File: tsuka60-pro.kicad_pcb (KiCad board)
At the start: 2 copper layers, 285 x 94.6 mm, 171 parts, among them J1 USB_C_Receptacle_USB2.0, J2 Conn_01x04_MountingPin, SW1 SW_Reset, U1 ATmega32U4-M, U2 SRV05-4, Y1 16MHz

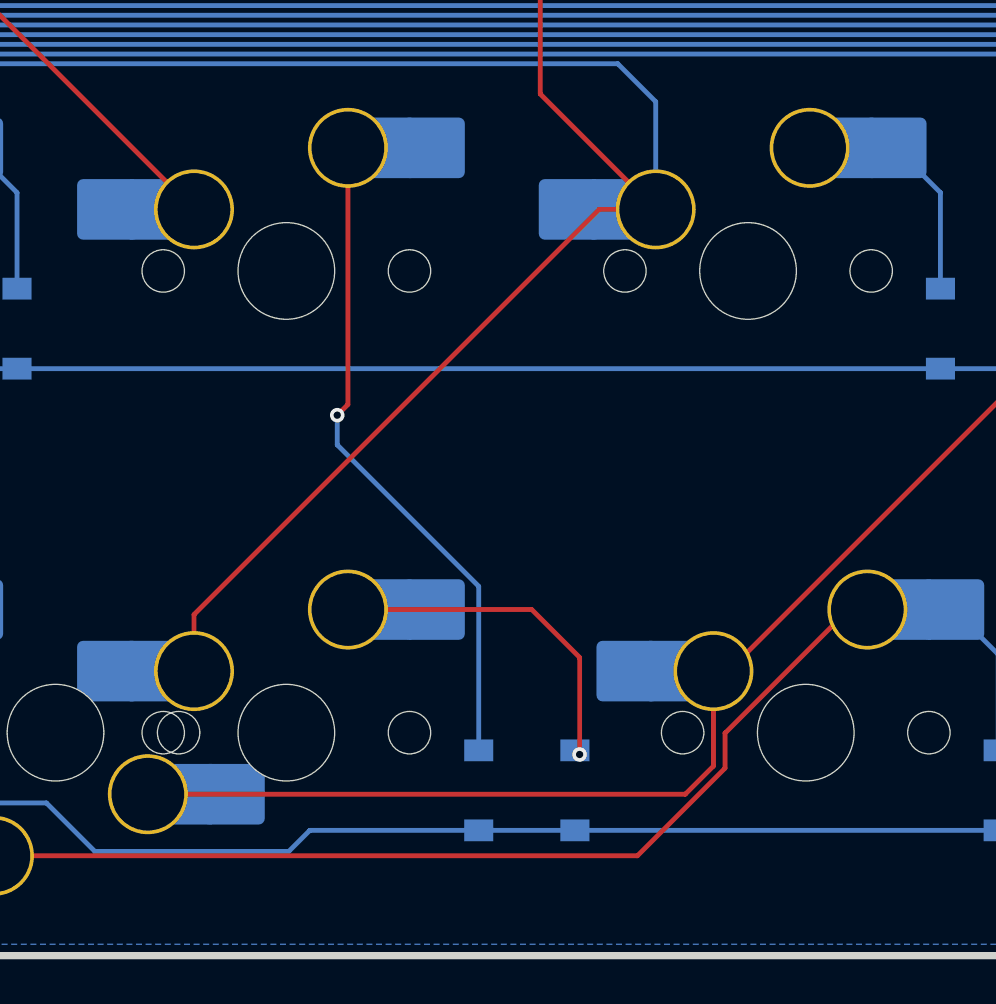
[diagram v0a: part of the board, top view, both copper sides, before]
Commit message: Update some traces
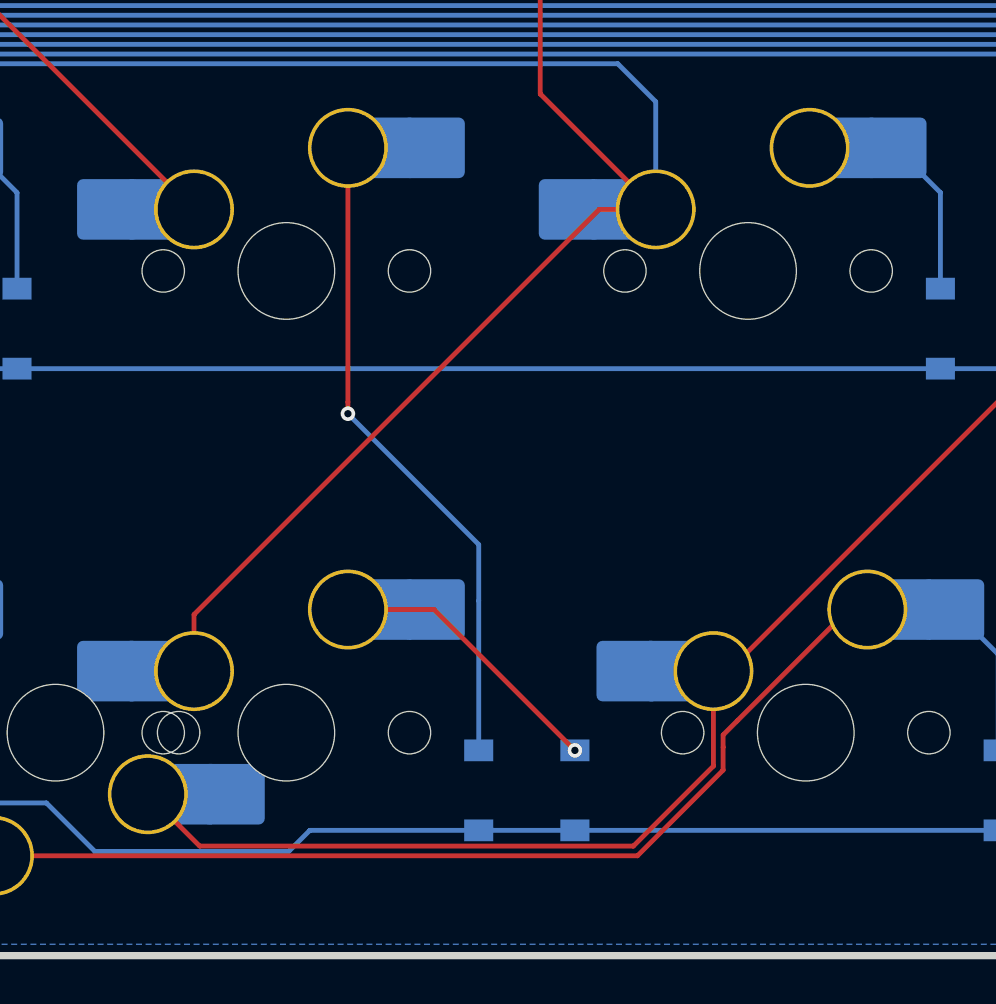
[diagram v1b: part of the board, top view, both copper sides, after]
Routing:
- net Net-(D69-Pad2): track 14.6 -> 11.8 mm
- net COL9: track 294.7 -> 296.4 mm
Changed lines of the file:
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@@
   (segment (start 187.325 161.922183) (end 187.325 165.83125) (width 0.2) (layer "B.Cu") (net 65))
   (segment (start 199.39 160.02) (end 189.227183 160.02) (width 0.2) (layer "B.Cu") (net 65))
-  (segment (start 218.44 151.56) (end 218 152) (width 0.2) (layer "F.Cu") (net 66))
-  (segment (start 218.44 140.97) (end 218.44 151.56) (width 0.2) (layer "F.Cu") (net 66))
-  (via (at 218 152) (size 0.6) (drill 0.3) (layers "F.Cu" "B.Cu") (net 66))
-  (segment (start 223.8375 165.83125) (end 223.8375 159.064683) (width 0.2) (layer "B.Cu") (net 66))
-  (segment (start 223.8375 159.064683) (end 218 153.227183) (width 0.2) (layer "B.Cu") (net 66))
-  (segment (start 218 153.227183) (end 218 152) (width 0.2) (layer "B.Cu") (net 66))
-  (segment (start 228 162) (end 226.02 160.02) (width 0.2) (layer "F.Cu") (net 67))
-  (segment (start 228 166) (end 228 162) (width 0.2) (layer "F.Cu") (net 67))
-  (segment (start 226.02 160.02) (end 218.44 160.02) (width 0.2) (layer "F.Cu") (net 67))
-  (via (at 228 166) (size 0.6) (drill 0.3) (layers "F.Cu" "B.Cu") (net 67))
-  (segment (start 227.83125 165.83125) (end 228 166) (width 0.2) (layer "B.Cu") (net 67))
-  (segment (start 227.80625 165.83125) (end 227.83125 165.83125) (width 0.2) (layer "B.Cu") (net 67))
+  (segment (start 218.44 140.97) (end 218.44 151.46) (width 0.2) (layer "F.Cu") (net 66))
+  (segment (start 218.44 151.46) (end 218.44 151.94) (width 0.2) (layer "F.Cu") (net 66))
+  (via (at 218.44 151.94) (size 0.6) (drill 0.3) (layers "F.Cu" "B.Cu") (net 66))
+  (segment (start 223.8375 165.83125) (end 223.8375 159.6625) (width 0.2) (layer "B.Cu") (net 66))
+  (segment (start 223.8375 157.3375) (end 218.44 151.94) (width 0.2) (layer "B.Cu") (net 66))
+  (segment (start 223.8375 159.6625) (end 223.8375 157.3375) (width 0.2) (layer "B.Cu") (net 66))
+  (segment (start 218.44 160.02) (end 221.995 160.02) (width 0.2) (layer "F.Cu") (net 67))
+  (segment (start 221.995 160.02) (end 227.80625 165.83125) (width 0.2) (layer "F.Cu") (net 67))
+  (via (at 227.80625 165.83125) (size 0.6) (drill 0.3) (layers "F.Cu" "B.Cu") (net 67))
   (segment (start 326.765 160.02) (end 328.6125 161.8675) (width 0.2) (layer "B.Cu") (net 68))
   (segment (start 328.6125 161.8675) (end 328.6125 165.83125) (width 0.2) (layer "B.Cu") (net 68))
@@
   (segment (start 94.065686 137.5) (end 229.575 137.5) (width 0.2) (layer "B.Cu") (net 79))
   (segment (start 240.665 86.36) (end 240.665 105.41) (width 0.2) (layer "F.Cu") (net 80))
+  (segment (start 233.52125 166.47875) (end 230.22 169.78) (width 0.2) (layer "F.Cu") (net 80))
   (segment (start 234.142414 162.56) (end 250.19 146.512414) (width 0.2) (layer "F.Cu") (net 80))
+  (segment (start 212.325 169.78) (end 210.185 167.64) (width 0.2) (layer "F.Cu") (net 80))
+  (segment (start 233.52125 162.56) (end 233.52125 166.47875) (width 0.2) (layer "F.Cu") (net 80))
   (segment (start 240.665 119.6975) (end 245.4275 124.46) (width 0.2) (layer "F.Cu") (net 80))
-  (segment (start 233.52125 166.47875) (end 233.52125 162.56) (width 0.2) (layer "F.Cu") (net 80))
   (segment (start 233.52125 162.56) (end 234.142414 162.56) (width 0.2) (layer "F.Cu") (net 80))
-  (segment (start 232.36 167.64) (end 233.52125 166.47875) (width 0.2) (layer "F.Cu") (net 80))
   (segment (start 245.4275 138.7475) (end 250.19 143.51) (width 0.2) (layer "F.Cu") (net 80))
   (segment (start 240.665 105.41) (end 240.665 119.6975) (width 0.2) (layer "F.Cu") (net 80))
-  (segment (start 210.185 167.64) (end 232.36 167.64) (width 0.2) (layer "F.Cu") (net 80))
+  (segment (start 230.22 169.78) (end 212.325 169.78) (width 0.2) (layer "F.Cu") (net 80))
   (segment (start 245.4275 124.46) (end 245.4275 138.7475) (width 0.2) (layer "F.Cu") (net 80))
   (segment (start 250.19 146.512414) (end 250.19 143.51) (width 0.2) (layer "F.Cu") (net 80))
@@
   (segment (start 183.35625 161.8675) (end 183.35625 165.83125) (width 0.2) (layer "B.Cu") (net 111))
   (segment (start 181.50875 160.02) (end 183.35625 161.8675) (width 0.2) (layer "B.Cu") (net 111))
-  (segment (start 234 165.116473) (end 234 166.565686) (width 0.2) (layer "F.Cu") (net 112))
-  (segment (start 239.096473 160.02) (end 234 165.116473) (width 0.2) (layer "F.Cu") (net 112))
-  (segment (start 234 166.565686) (end 230.385686 170.18) (width 0.2) (layer "F.Cu") (net 112))
+  (segment (start 239.096473 160.02) (end 234.508236 164.608236) (width 0.2) (layer "F.Cu") (net 112))
+  (segment (start 234.508236 164.608236) (end 233.92125 165.195222) (width 0.2) (layer "F.Cu") (net 112))
+  (segment (start 233.92125 166.644436) (end 230.385686 170.18) (width 0.2) (layer "F.Cu") (net 112))
+  (segment (start 233.92125 165.195222) (end 233.92125 165.7) (width 0.2) (layer "F.Cu") (net 112))
+  (segment (start 233.92125 165.7) (end 233.92125 166.644436) (width 0.2) (layer "F.Cu") (net 112))
   (segment (start 239.87125 160.02) (end 239.096473 160.02) (width 0.2) (layer "F.Cu") (net 112))
   (segment (start 230.385686 170.18) (end 203.835 170.18) (width 0.2) (layer "F.Cu") (net 112))
